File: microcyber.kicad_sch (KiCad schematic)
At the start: 10 parts

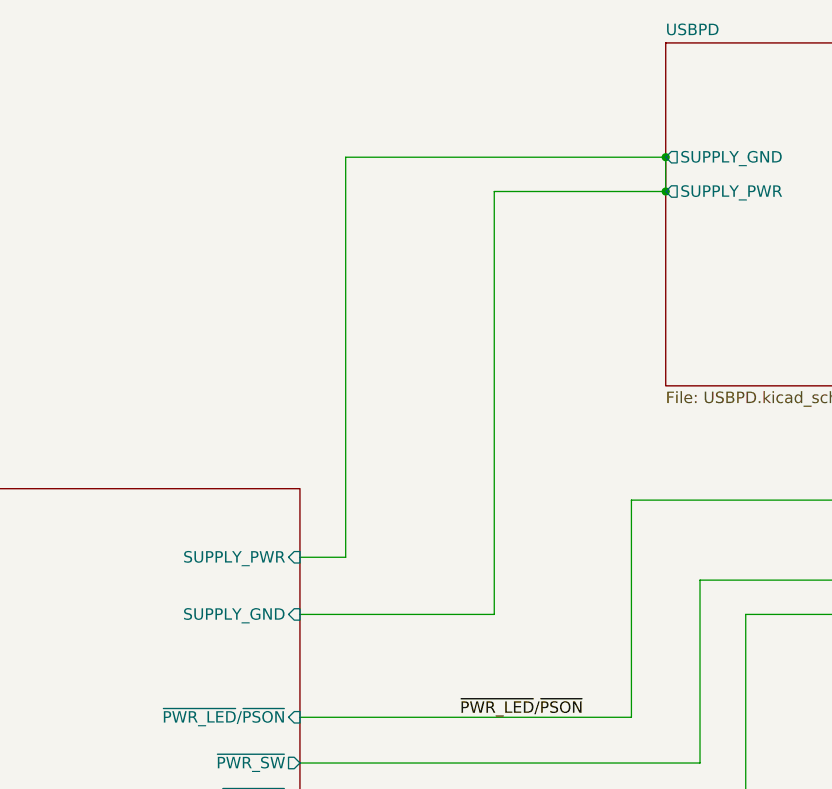
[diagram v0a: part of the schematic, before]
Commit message: before board exclusion
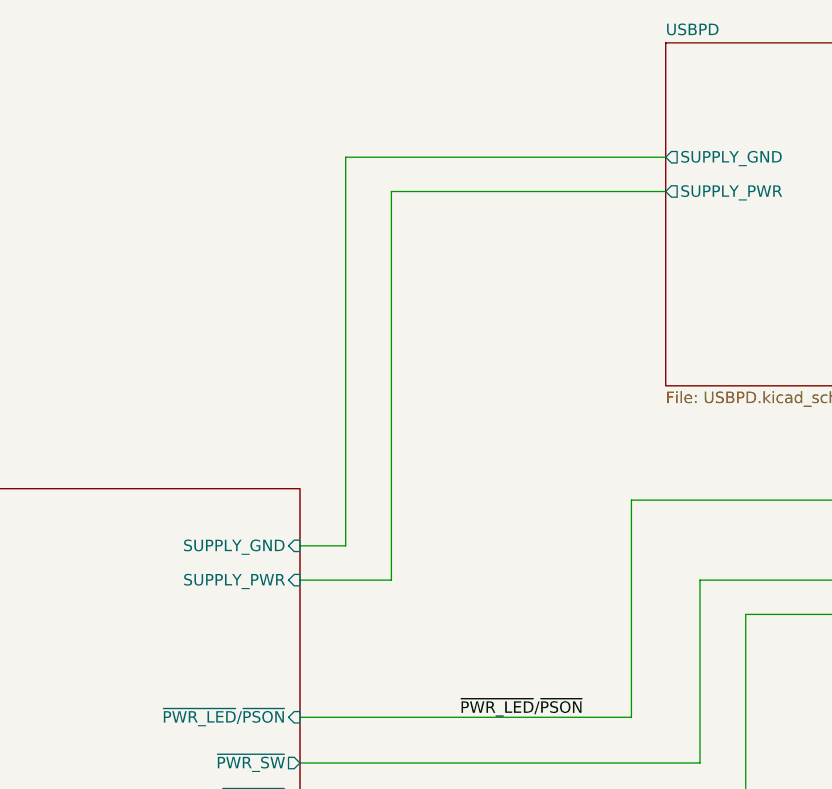
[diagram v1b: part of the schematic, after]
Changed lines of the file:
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@@
 	)
 	(junction
-		(at 123.19 26.67)
-		(diameter 0)
-		(color 0 0 0 0)
-	)
-	(junction
-		(at 123.19 30.48)
-		(diameter 0)
-		(color 0 0 0 0)
-	)
-	(junction
 		(at 425.45 334.01)
 		(diameter 0)
@@
 	(wire
 		(pts
-			(xy 123.19 30.48) (xy 123.19 26.67)
-		)
-		(stroke
-			(width 0)
-			(type default)
-		)
-	)
-	(wire
-		(pts
 			(xy 158.75 168.91) (xy 177.8 168.91)
 		)
@@
 	(wire
 		(pts
-			(xy 82.55 71.12) (xy 87.63 71.12)
-		)
-		(stroke
-			(width 0)
-			(type default)
-		)
-	)
-	(wire
-		(pts
 			(xy 127 73.66) (xy 127 93.98)
 		)
@@
 	(wire
 		(pts
+			(xy 82.55 73.66) (xy 92.71 73.66)
+		)
+		(stroke
+			(width 0)
+			(type default)
+		)
+	)
+	(wire
+		(pts
 			(xy 158.75 186.69) (xy 189.23 186.69)
 		)
@@
 	(wire
 		(pts
+			(xy 92.71 30.48) (xy 92.71 73.66)
+		)
+		(stroke
+			(width 0)
+			(type default)
+		)
+	)
+	(wire
+		(pts
 			(xy 331.47 243.84) (xy 347.98 243.84)
 		)
@@
 	(wire
 		(pts
+			(xy 82.55 69.85) (xy 87.63 69.85)
+		)
+		(stroke
+			(width 0)
+			(type default)
+		)
+	)
+	(wire
+		(pts
 			(xy 331.47 229.87) (xy 347.98 229.87)
 		)
@@
 	(wire
 		(pts
-			(xy 87.63 26.67) (xy 87.63 71.12)
+			(xy 87.63 26.67) (xy 87.63 69.85)
 		)
 		(stroke
@@
 	(wire
 		(pts
-			(xy 104.14 30.48) (xy 123.19 30.48)
-		)
-		(stroke
-			(width 0)
-			(type default)
-		)
-	)
-	(wire
-		(pts
 			(xy 407.67 317.5) (xy 429.26 317.5)
 		)
@@
 	(wire
 		(pts
-			(xy 104.14 30.48) (xy 104.14 77.47)
-		)
-		(stroke
-			(width 0)
-			(type default)
-		)
-	)
-	(wire
-		(pts
 			(xy 331.47 318.77) (xy 345.44 318.77)
 		)
@@
 	(wire
 		(pts
-			(xy 445.77 336.55) (xy 425.45 336.55)
+			(xy 92.71 30.48) (xy 123.19 30.48)
 		)
 		(stroke
@@
 	(wire
 		(pts
-			(xy 104.14 77.47) (xy 82.55 77.47)
+			(xy 445.77 336.55) (xy 425.45 336.55)
 		)
 		(stroke
@@
 		(in_bom yes)
 		(on_board yes)
-		(dnp no)
+		(dnp yes)
 		(fields_autoplaced yes)
 		(stroke
@@
 		(in_bom yes)
 		(on_board yes)
-		(dnp no)
+		(dnp yes)
 		(fields_autoplaced yes)
 		(stroke
@@
 		)
 		(pin "SUPPLY_GND" input
-			(at 82.55 77.47 0)
+			(at 82.55 69.85 0)
 			(effects
 				(font
@@
 		)
 		(pin "SUPPLY_PWR" input
-			(at 82.55 71.12 0)
+			(at 82.55 73.66 0)
 			(effects
 				(font
